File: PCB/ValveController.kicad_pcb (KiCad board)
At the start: 2 copper layers, 50 x 50 mm, 39 parts, among them J1 Conn_01x04, J2 TTP224, J3 Valve 1, J4 Valve 2, J5 Input 24V, J6 4-20 IO, Q1 30N06, Q2 30N06, Q3 2N7002, Q4 AO3401A, Q5 2N7002, Q6 SI2319A, Q7 BC807, U1 ESP32-C3-SuperMini, U2 XTR111AxDGQ, U3 MCP4725xxx-xCH, U4 UMW_78M05_TO252, U5 PCF8574DWR

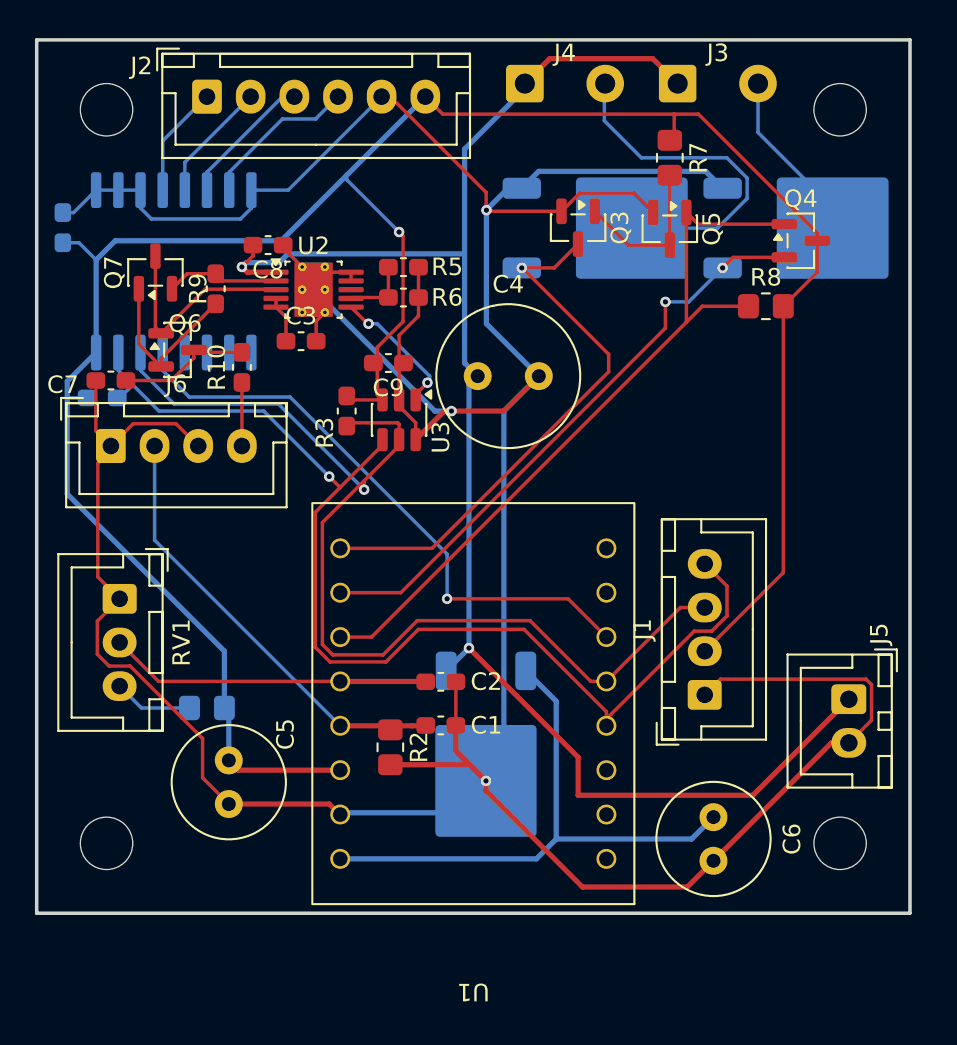
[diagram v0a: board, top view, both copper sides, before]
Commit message: refactoring
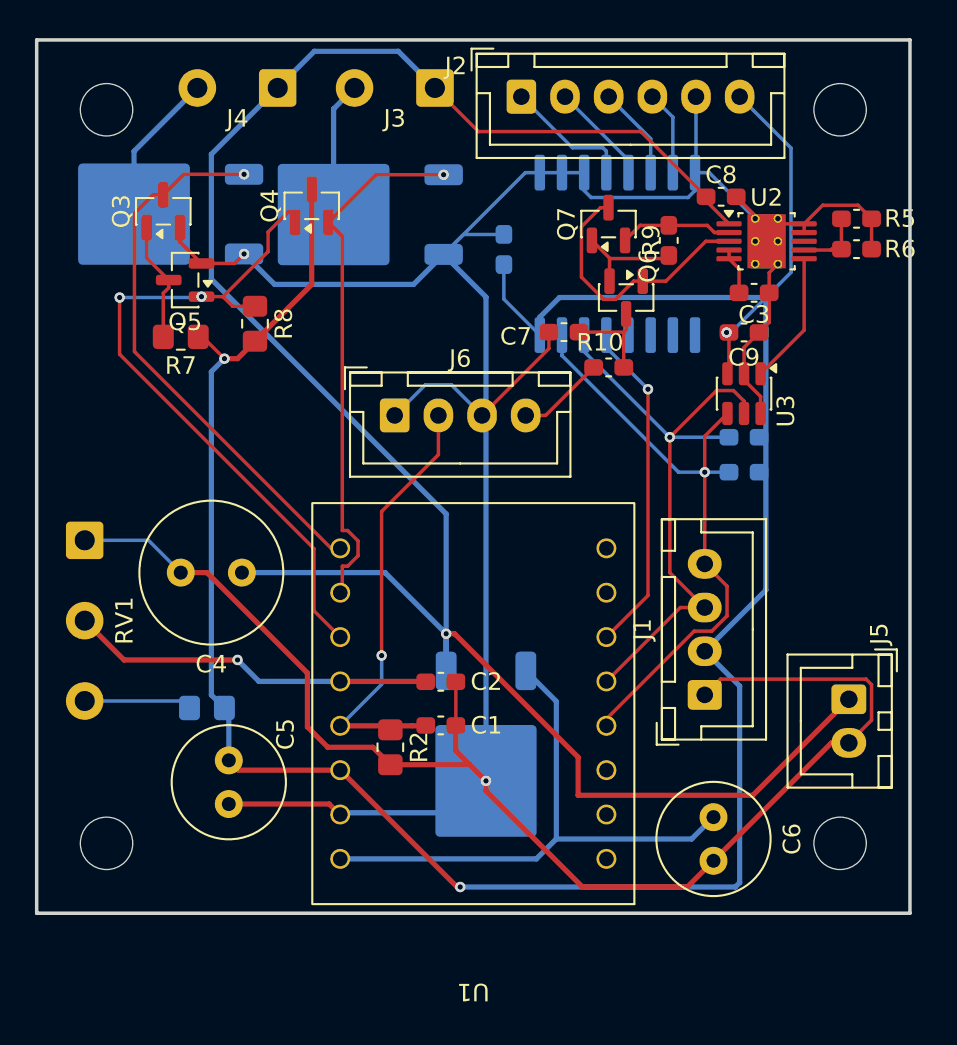
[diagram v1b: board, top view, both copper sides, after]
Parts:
- R3: moved to B.Cu
- RV1: footprint Connector_JST:JST_XH_B3B-XH-A_1x03_P2.50mm_Vertical -> Connector_Wire:SolderWire-0.5sqmm_1x03_P4.6mm_D0.9mm_OD2.1mm
- moved R4 37.0 mm to (90.5, 74.8), turned to 180 degrees
- moved R7 29.8 mm to (58.2, 67.0), turned to 180 degrees
- moved R8 29.3 mm to (62.5, 66.2), turned to -90 degrees
- moved Q4 28.1 mm to (65.8, 59.5), turned to 90 degrees
- moved Q5 27.9 mm to (58.5, 63.8), turned to 180 degrees
- moved U2 26.1 mm to (91.8, 61.5)
- moved C3 26.1 mm to (91.1, 64.5)
- moved C7 26.1 mm to (80.2, 66.7)
- moved C8 26.1 mm to (89.2, 59.0)
- moved Q7 26.1 mm to (82.7, 60.5)
- moved R5 26.1 mm to (96.9, 60.2)
- moved R6 26.1 mm to (96.9, 62.0)
- moved R9 26.1 mm to (86.2, 61.5)
- moved Q1 26.1 mm to (68.3, 60.0), turned to 180 degrees
- moved Q2 26.0 mm to (56.8, 60.0), turned to 180 degrees
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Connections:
- net Net-(J1-Pin_3) renamed /I2C_SCL
- net Net-(J1-Pin_4) renamed /I2C_SDA
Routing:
- net /I2C_SDA: track 64.8 -> 36.0 mm
- net GNDPWR: track 233.5 -> 205.8 mm, vias 3 -> 2
- net +24V: track 91.5 -> 117.2 mm, vias 2 -> 1
- net /I2C_SCL: track 60.4 -> 35.5 mm
- net Net-(U1-GPIO10): track 34.3 -> 19.3 mm
- net Net-(J4-Pin_2): track 20.2 -> 8.73 mm
- net +3.3V: track 136.2 -> 144.2 mm, vias 1 -> 3
- net Net-(J2-Pin_4): track 9.04 -> 4.84 mm
- net Net-(Q1-G): track 34.3 -> 30.4 mm, vias 2 -> 1
- net Net-(Q4-G): track 43.4 -> 39.7 mm, vias 0 -> 2
- net Net-(Q6-S): track 9.86 -> 6.21 mm
- net Net-(Q6-G): track 12.2 -> 15.2 mm
- net Net-(U1-GPIO3): track 18.5 -> 21.0 mm, vias 0 -> 1
- net Net-(J2-Pin_3): track 7.81 -> 5.35 mm
- net Net-(J3-Pin_2): track 10.0 -> 7.75 mm
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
